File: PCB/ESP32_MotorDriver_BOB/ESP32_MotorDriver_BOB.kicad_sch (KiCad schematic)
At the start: 39 parts, among them J1 USB_C_Receptacle_USB2.0, J2 Conn_01x06, J3 Conn_01x06, J5 Conn_01x18, J6 Conn_01x07, Q1 SSM3J338R_LF, SW1 EN, SW2 BOOT, U1 ESP32-S2-SOLO-N4, U2 D3V3XA4B10LP, U4 TB6612FNG, U5 AP63203WU

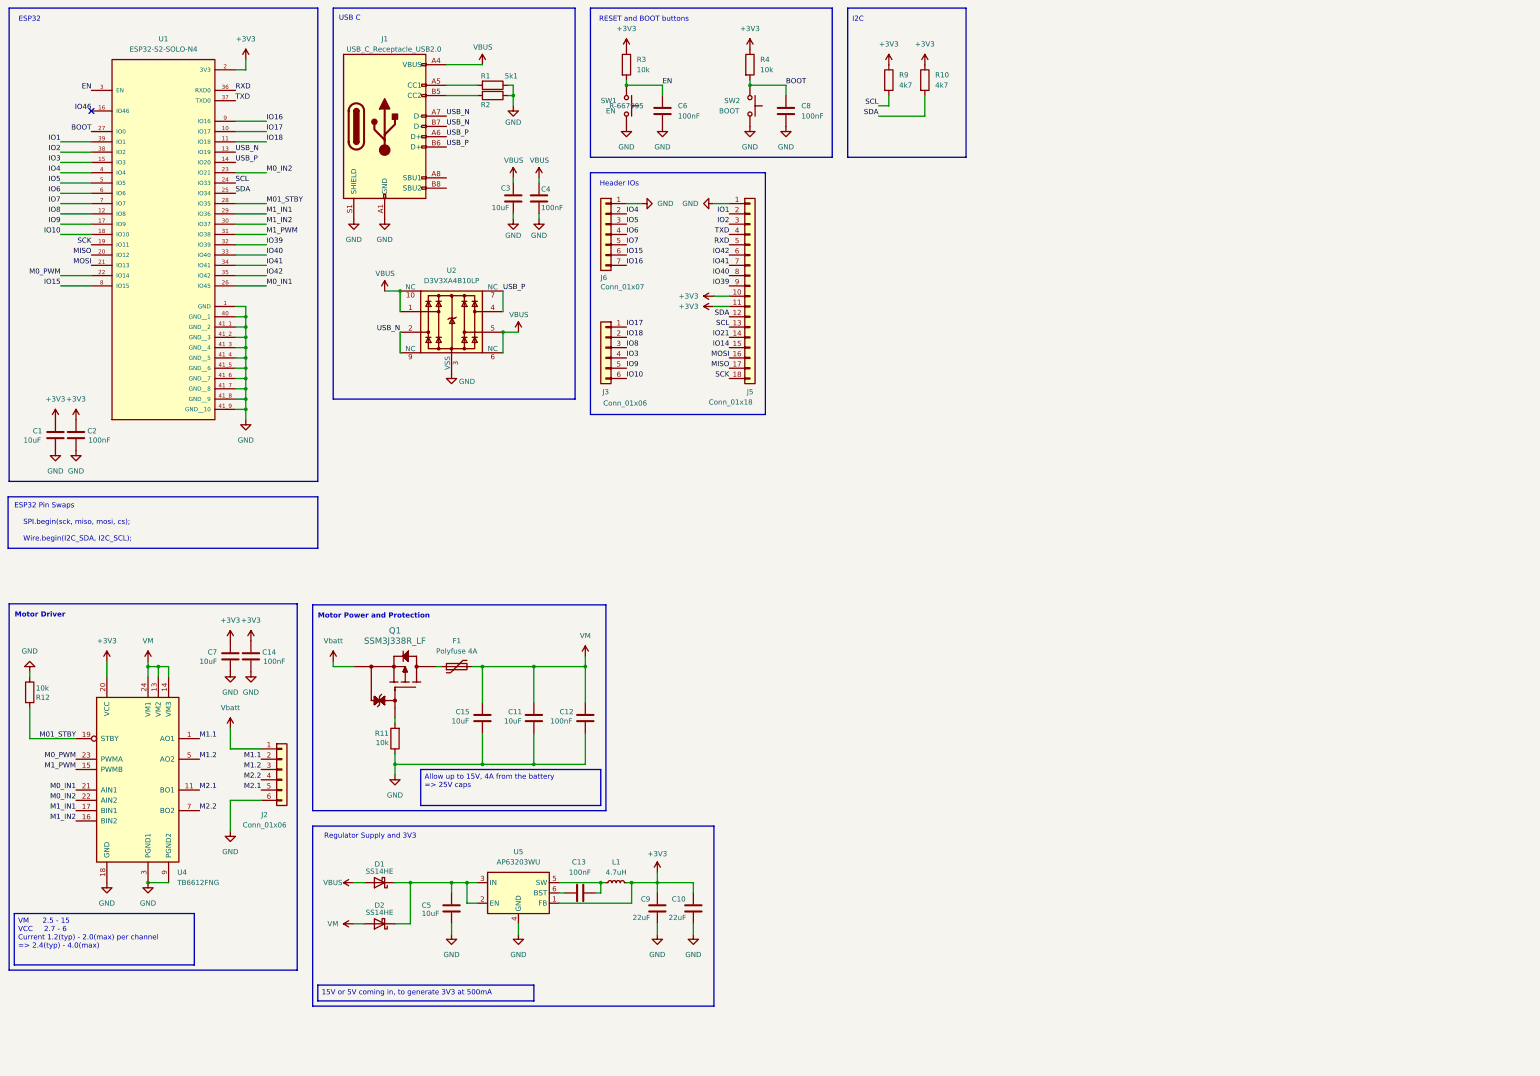
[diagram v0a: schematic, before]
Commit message: actual _v01
Issue with files being copied - these should be good
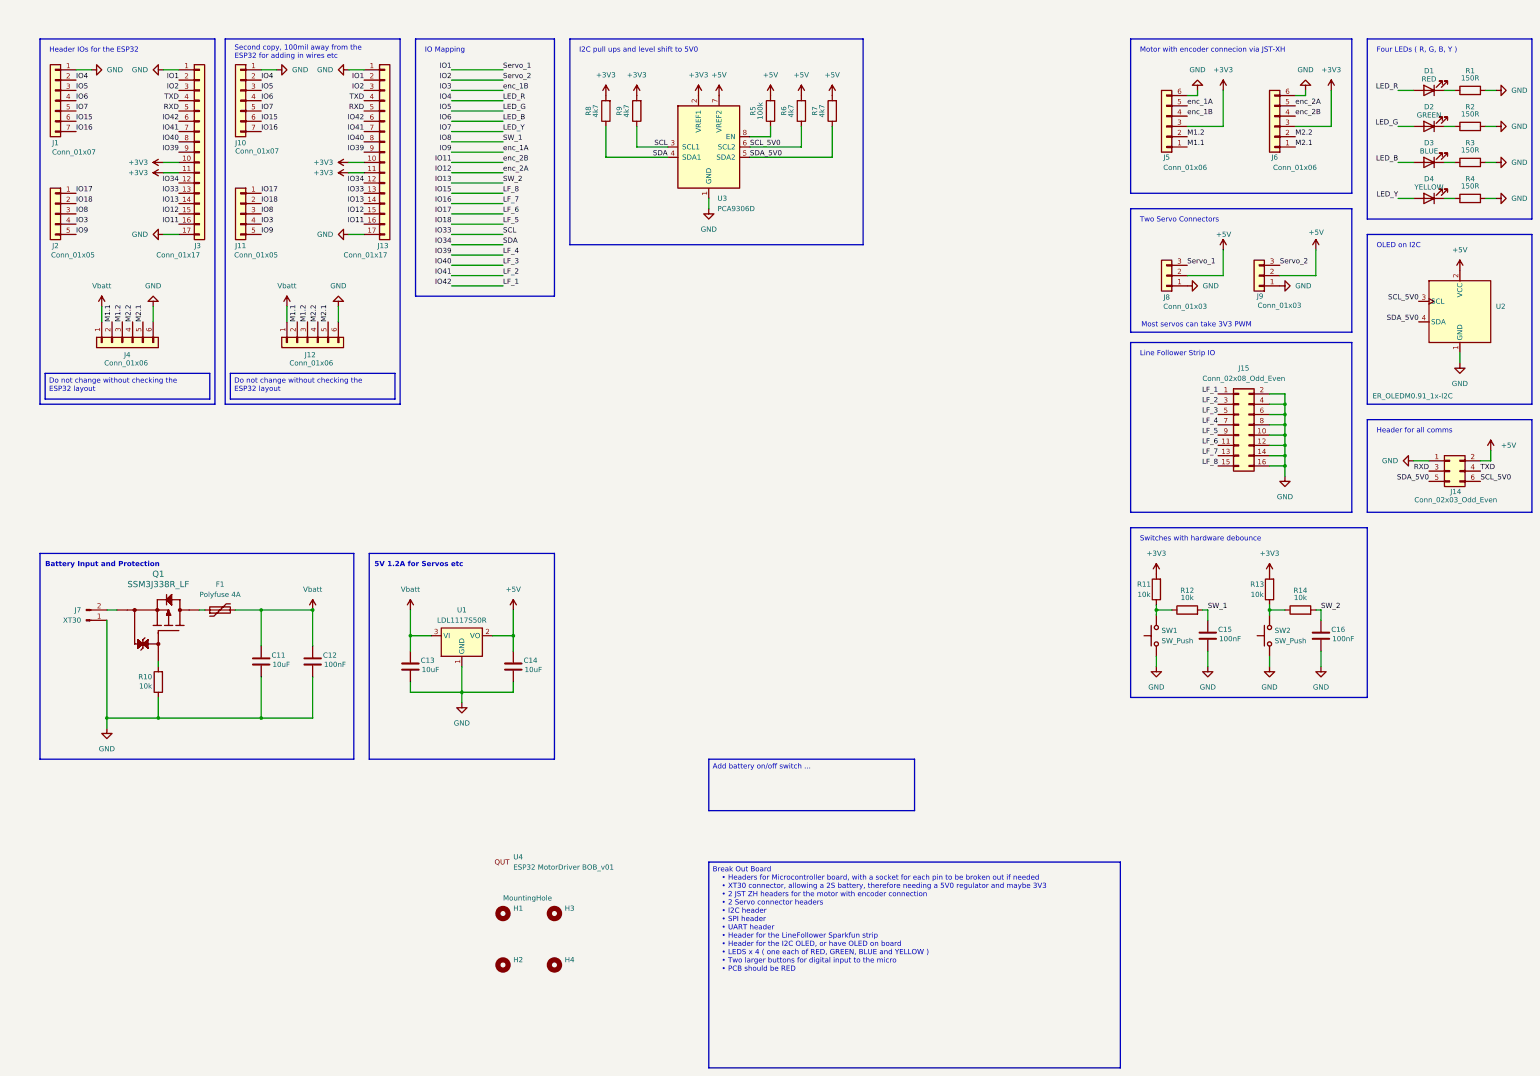
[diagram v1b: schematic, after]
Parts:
- removed C1, C3, C5, C7: 10uF, Capacitor_SMD:C_0805_2012Metric_Pad1.18x1.45mm_HandSolder, symbol Device:C
- removed C10, C9: 22uF, Capacitor_SMD:C_0805_2012Metric_Pad1.18x1.45mm_HandSolder, symbol Device:C
- removed C2, C4, C6, C8: 100nF, Capacitor_SMD:C_0402_1005Metric_Pad0.74x0.62mm_HandSolder, symbol Device:C
- removed D1, D2: D_Schottky, Diode_SMD:D_SOD-323F, symbol Device:D_Schottky
- removed J1: USB_C_Receptacle_USB2.0, Connector_USB:USB_C_Receptacle_HRO_TYPE-C-31-M-12, symbol Connector:USB_C_Receptacle_USB2.0
- removed J2, J3: Conn_01x06, Connector_PinHeader_2.54mm:PinHeader_1x06_P2.54mm_Vertical, symbol Connector_Generic:Conn_01x06
- removed J5: Conn_01x18, Connector_PinHeader_2.54mm:PinHeader_1x18_P2.54mm_Vertical, symbol Connector_Generic:Conn_01x18
- removed L1: 4.7uH, Inductor_SMD:L_1008_2520Metric_Pad1.43x2.20mm_HandSolder, symbol Device:L_Small
- removed U1: ESP32-S2-SOLO-N4, ESP32_S2_SOLO_N4:XCVR_ESP32-S2-SOLO-N4, symbol ESP32-S2-SOLO-N4:ESP32-S2-SOLO-N4
- removed U2: D3V3XA4B10LP, Package_DFN_QFN:Diodes_UDFN-10_1x2.5mm_P0.5mm, symbol Power_Protection:D3V3XA4B10LP
- removed U4: TB6612FNG, Package_SO:SSOP-24_5.3x8.2mm_P0.65mm, symbol Driver_Motor:TB6612FNG
- removed U5: AP63203WU, Package_TO_SOT_SMD:TSOT-23-6, symbol Regulator_Switching:AP63203WU
- added C16: 100nF, Capacitor_SMD:C_0402_1005Metric_Pad0.74x0.62mm_HandSolder, symbol Device:C
- added D1: RED, LED_SMD:LED_1206_3216Metric_Pad1.42x1.75mm_HandSolder, symbol Device:LED
- added D2: GREEN, LED_SMD:LED_1206_3216Metric_Pad1.42x1.75mm_HandSolder, symbol Device:LED
- added D3: BLUE, LED_SMD:LED_1206_3216Metric_Pad1.42x1.75mm_HandSolder, symbol Device:LED
- added D4: YELLOW, LED_SMD:LED_1206_3216Metric_Pad1.42x1.75mm_HandSolder, symbol Device:LED
- added H1, H2, H3, H4: MountingHole, MountingHole:MountingHole_3.2mm_M3, symbol Mechanical:MountingHole
- added J10: Conn_01x07, Connector_PinSocket_2.54mm:PinSocket_1x07_P2.54mm_Vertical, symbol Connector_Generic:Conn_01x07
- added J11, J2: Conn_01x05, Connector_PinSocket_2.54mm:PinSocket_1x05_P2.54mm_Vertical, symbol Connector_Generic:Conn_01x05
- added J12, J4: Conn_01x06, Connector_PinSocket_2.54mm:PinSocket_1x06_P2.54mm_Vertical, symbol Connector_Generic:Conn_01x06
- added J13, J3: Conn_01x17, Connector_PinSocket_2.54mm:PinSocket_1x17_P2.54mm_Vertical, symbol Connector_Generic:Conn_01x17
- added J14: Conn_02x03_Odd_Even, Connector_PinHeader_2.54mm:PinHeader_2x03_P2.54mm_Vertical, symbol Connector_Generic:Conn_02x03_Odd_Even
- added J15: Conn_02x08_Odd_Even, Connector_PinHeader_2.54mm:PinHeader_2x08_P2.54mm_Vertical, symbol Connector_Generic:Conn_02x08_Odd_Even
- added J5, J6: Conn_01x06, Connector_JST:JST_XH_S6B-XH-A_1x06_P2.50mm_Horizontal, symbol Connector_Generic:Conn_01x06
- added J7: XT30, Connector_AMASS:AMASS_XT30PW-M_1x02_P2.50mm_Horizontal, symbol Connector:Conn_01x02_Pin
- added J8, J9: Conn_01x03, Connector_PinHeader_2.54mm:PinHeader_1x03_P2.54mm_Vertical, symbol Connector_Generic:Conn_01x03
- added R13, R14: 10k, Resistor_SMD:R_0402_1005Metric_Pad0.72x0.64mm_HandSolder, symbol Device:R
- added R5: 100k, Resistor_SMD:R_0402_1005Metric_Pad0.72x0.64mm_HandSolder, symbol Device:R
- added R6, R7, R8: 4k7, Resistor_SMD:R_0402_1005Metric_Pad0.72x0.64mm_HandSolder, symbol Device:R
- added U1: LDL1117S50R, Package_TO_SOT_SMD:SOT-223-3_TabPin2, symbol Regulator_Linear:LD1117S50TR_SOT223
- added U2: ER_OLEDM0.91_1x-I2C, Display:ER_OLEDM0.91_1x-I2C, symbol Display_Graphic:ER_OLEDM0.91_1x-I2C
- added U3: PCA9306D, Package_SO:SO-8_3.9x4.9mm_P1.27mm, symbol Interface:PCA9306D
- added U4: ESP32 MotorDriver BOB_v01, _silkscreen:logo_QUT, symbol _silkscreen:logo_qut
- C11: footprint Capacitor_SMD:C_0805_2012Metric_Pad1.18x1.45mm_HandSolder -> Capacitor_SMD:C_0402_1005Metric_Pad0.74x0.62mm_HandSolder; Manufacturer (none) -> Samsung Electro-Mechanics; PN_Digikey (none) -> 1276-CL05A106MP6NUN8CT-ND; PN_LCSC (none) -> C3902158; PN_Manufacturer (none) -> CL05A106MP6NUN8
- C12: Manufacturer (none) -> YAGEO; PN_Digikey (none) -> 311-3342-1-ND; PN_LCSC (none) -> C105882; PN_Manufacturer (none) -> CC0402KRX5R9BB104
- C13: value 100nF -> 10uF; LCSC PN C105882 -> C3902158; Manufacturer (none) -> Samsung Electro-Mechanics; PN_Digikey (none) -> 1276-CL05A106MP6NUN8CT-ND; PN_LCSC (none) -> C3902158; PN_Manufacturer (none) -> CL05A106MP6NUN8
- C14: value 100nF -> 10uF; LCSC PN (none) -> C3902158; Manufacturer (none) -> Samsung Electro-Mechanics; PN_Digikey (none) -> 1276-CL05A106MP6NUN8CT-ND; PN_LCSC (none) -> C3902158; PN_Manufacturer (none) -> CL05A106MP6NUN8
- C15: value 10uF -> 100nF; footprint Capacitor_SMD:C_0805_2012Metric_Pad1.18x1.45mm_HandSolder -> Capacitor_SMD:C_0402_1005Metric_Pad0.74x0.62mm_HandSolder; LCSC PN (none) -> C105882; Manufacturer (none) -> YAGEO; PN_Digikey (none) -> 311-3342-1-ND; PN_LCSC (none) -> C105882; PN_Manufacturer (none) -> CC0402KRX5R9BB104
- F1: footprint Fuse:Fuse_0805_2012Metric_Pad1.15x1.40mm_HandSolder -> digikey-footprints:0805; Manufacturer (none) -> Vishay
- J1: renamed from J6; footprint Connector_PinHeader_2.54mm:PinHeader_1x07_P2.54mm_Vertical -> Connector_PinSocket_2.54mm:PinSocket_1x07_P2.54mm_Vertical
- Q1: footprint SSM3J338R_LF:SOT-23F_TOS -> SSM3J338R:SOT-23F_TOS; Manufacturer (none) -> Toshiba Semiconductor and Storage
- R1, R2: value 5k1 -> 150R
- R10: value 4k7 -> 10k; LCSC PN (none) -> C851816; LCSC Part # C100047 -> (none); Manufacturer (none) -> YAGEO; PN_Digikey (none) -> YAG1249CT-ND; PN_LCSC (none) -> C851816; PN_Manufacturer (none) -> RC0402FR-0710KP
- R11, R12: LCSC PN C851816 -> (none)
- R3, R4: value 10k -> 150R; LCSC Part # C100047 -> (none)
- R9: LCSC Part # C100047 -> (none)
- SW1: value EN -> SW_Push; footprint _common:Switch SMD STO -> Button_Switch_SMD:SW_SPST_EVQP0; PN_Digikey 2508-R-667995CT-ND -> P12966SCT-ND; PN_Manufacturer R-667995 -> (none)
- SW2: value BOOT -> SW_Push; footprint _common:Switch SMD STO -> Button_Switch_SMD:SW_SPST_EVQP0; LCSC_PN C25168823 -> (none); PN_Digikey 2508-R-667995CT-ND -> P12966SCT-ND; PN_Manufacturer R-667995 -> (none)
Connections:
- net BOOT is gone; now on net GND: R4.2, SW2.1
- net EN is gone; now on net GND: R3.2, SW1.1
- net M01_STBY is gone; now on net IO8: R12.2
- net SCL is gone; now on net +3V3: R9.2
- net SDA is gone; now on an unnamed net: R10.2
- net +3V3: now also R11.2, J13.10 (Pin_10), J13.11 (Pin_11), J3.10 (Pin_10), J3.11 (Pin_11), J5.3 (Pin_3), J6.3 (Pin_3), R13.2, R8.2, U3.2 (VREF1); no longer C14.1, R10.1, R3.1, R4.1, R9.1
- net GND: now also C13.2, R1.2, R10.1, R2.2, C16.2, J10.1 (Pin_1), J12.6 (Pin_6), J13.1 (Pin_1), J13.17 (Pin_17), J14.1 (Pin_1), J15.10 (Pin_10), J15.12 (Pin_12), J15.14 (Pin_14), J15.16 (Pin_16), J15.2 (Pin_2), J15.4 (Pin_4), J15.6 (Pin_6), J15.8 (Pin_8), J3.1 (Pin_1), J3.17 (Pin_17), J4.6 (Pin_6), J5.6 (Pin_6), J6.6 (Pin_6), J7.1 (Pin_1), J8.1 (Pin_1), J9.1 (Pin_1), U1.1 (GND), U2.1 (GND), U3.1 (GND); no longer R1.1, R11.1, R12.1, R2.1, SW1.2, SW2.2
- net IO1: now also J13.2 (Pin_2), J3.2 (Pin_2), J8.3 (Pin_3)
- net IO15: now also J10.6 (Pin_6), J15.15 (Pin_15)
- net IO16: now also J10.7 (Pin_7), J15.13 (Pin_13)
- net IO17: now also J11.1 (Pin_1), J15.11 (Pin_11), J2.1 (Pin_1)
- net IO18: now also J11.2 (Pin_2), J15.9 (Pin_9), J2.2 (Pin_2)
- net IO2: now also J13.3 (Pin_3), J3.3 (Pin_3), J9.3 (Pin_3)
- net IO3: now also J11.4 (Pin_4), J2.4 (Pin_4), J5.4 (Pin_4)
- net IO39: now also J13.9 (Pin_9), J15.7 (Pin_7), J3.9 (Pin_9)
- net IO4: now also D1.2 (A), J10.2 (Pin_2)
- net IO40: now also J13.8 (Pin_8), J15.5 (Pin_5), J3.8 (Pin_8)
- net IO41: now also J13.7 (Pin_7), J15.3 (Pin_3), J3.7 (Pin_7)
- net IO42: now also J13.6 (Pin_6), J15.1 (Pin_1), J3.6 (Pin_6)
- net IO5: now also D2.2 (A), J10.3 (Pin_3)
- net IO6: now also D3.2 (A), J10.4 (Pin_4)
- net IO7: now also D4.2 (A), J10.5 (Pin_5)
- net IO8: now also C15.1, J11.3 (Pin_3), J2.3 (Pin_3)
- net IO9: now also J11.5 (Pin_5), J2.5 (Pin_5), J5.5 (Pin_5)
- net M1.1: now also J12.2 (Pin_2), J4.2 (Pin_2), J5.1 (Pin_1)
- net M1.2: now also J12.3 (Pin_3), J4.3 (Pin_3), J5.2 (Pin_2)
- net M2.1: now also J12.5 (Pin_5), J4.5 (Pin_5), J6.1 (Pin_1)
- net M2.2: now also J12.4 (Pin_4), J4.4 (Pin_4), J6.2 (Pin_2)
- net RXD: now also J13.5 (Pin_5), J14.3 (Pin_3), J3.5 (Pin_5)
- net TXD: now also J13.4 (Pin_4), J14.4 (Pin_4), J3.4 (Pin_4)
- net Vbatt: now also C11.1, C12.1, C13.1, F1.2, J12.1 (Pin_1), J4.1 (Pin_1), U1.3 (VI); no longer Q1.2
- net at Q1.1: no longer R11.2
- removed net VM: C11.1, C12.1, C15.1, F1.2
- new net: D2.1 (K), R2.1
- new net: D4.1 (K), R4.1
- new net: R13.1, R14.1, SW2.2
- new net: R11.1, R12.1, SW1.2
- new net: R5.1, U3.8 (EN)
- new net: D3.1 (K), R3.1
- new net: J7.2 (Pin_2), Q1.2
- new net: D1.1 (K), R1.1
- new net +5V: C14.1, J14.2 (Pin_2), J8.2 (Pin_2), J9.2 (Pin_2), R5.2, R6.2, R7.2, U1.2 (VO), U2.2 (VCC), U3.7 (VREF2)
- new net IO11: J13.16 (Pin_16), J3.16 (Pin_16), J6.4 (Pin_4)
- new net IO12: J13.15 (Pin_15), J3.15 (Pin_15), J6.5 (Pin_5)
- new net IO13: C16.1, J13.14 (Pin_14), J3.14 (Pin_14), R14.2
- new net IO33: J13.13 (Pin_13), J3.13 (Pin_13), R9.1, U3.3 (SCL1)
- new net IO34: J13.12 (Pin_12), J3.12 (Pin_12), R8.1, U3.4 (SDA1)
- new net SCL_5V0: J14.6 (Pin_6), R6.1, U2.3 (SCL), U3.6 (SCL2)
- new net SDA_5V0: J14.5 (Pin_5), R7.1, U2.4 (SDA), U3.5 (SDA2)
- no-connect marks 1 -> 0
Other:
- note added: "5V 1.2A for Servos etc"
- note added: "Battery Input and Protection"
- note added: "Four LEDs ( R, G, B, Y )"
- note added: "Header IOs for the ESP32"
- note added: "Header for all comms"
- note added: "I2C pull ups and level shift to 5V0"
- note added: "IO Mapping"
- note added: "Line Follower Strip IO"
- note added: "Most servos can take 3V3 PWM"
- note added: "Motor with encoder connecion via JST-XH"
- note added: "OLED on I2C"
- note added: "Second copy, 100mil away from the ESP32 for adding in wires etc"
- note added: "Switches with hardware debounce"
- note added: "Two Servo Connectors"
- note removed: "ESP32"
- note removed: "ESP32 Pin Swaps SPI.begin(sck, miso, mosi, cs); Wire.begin(I2C_SDA, I2C_SCL);"
- note removed: "Header IOs"
- note removed: "I2C"
- note removed: "Motor Driver"
- note removed: "Motor Power and Protection"
- note removed: "RESET and BOOT buttons"
- note removed: "Regulator Supply and 3V3"
- note removed: "USB C"
- moved on the sheet: J1
